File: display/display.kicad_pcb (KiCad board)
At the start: 2 copper layers, 177 x 107.2 mm, 19 parts, among them J1 DIN41612_03x32_ABC

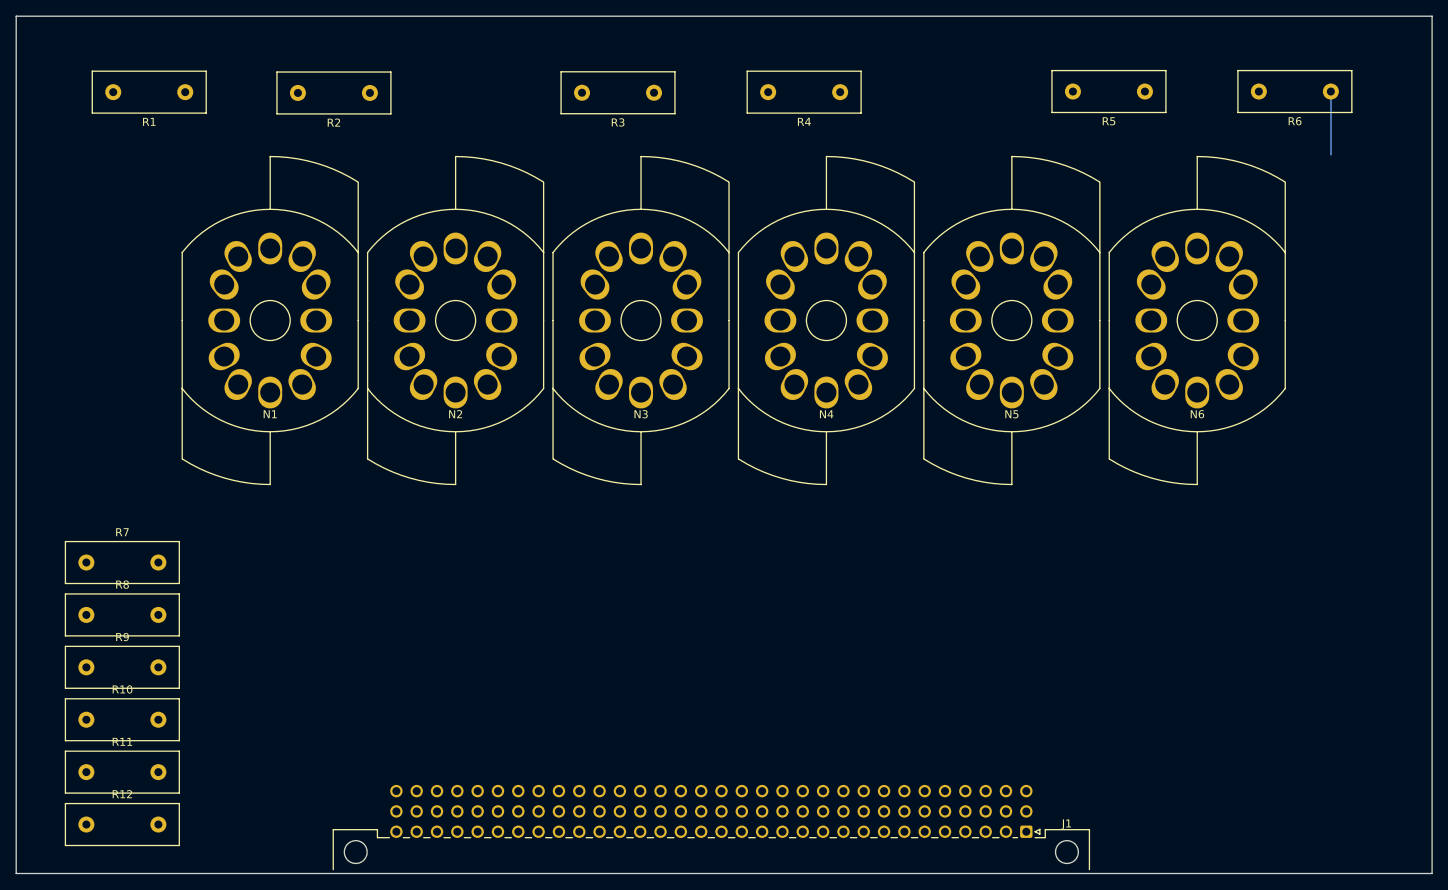
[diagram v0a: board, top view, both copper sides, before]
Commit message: Ongoing development
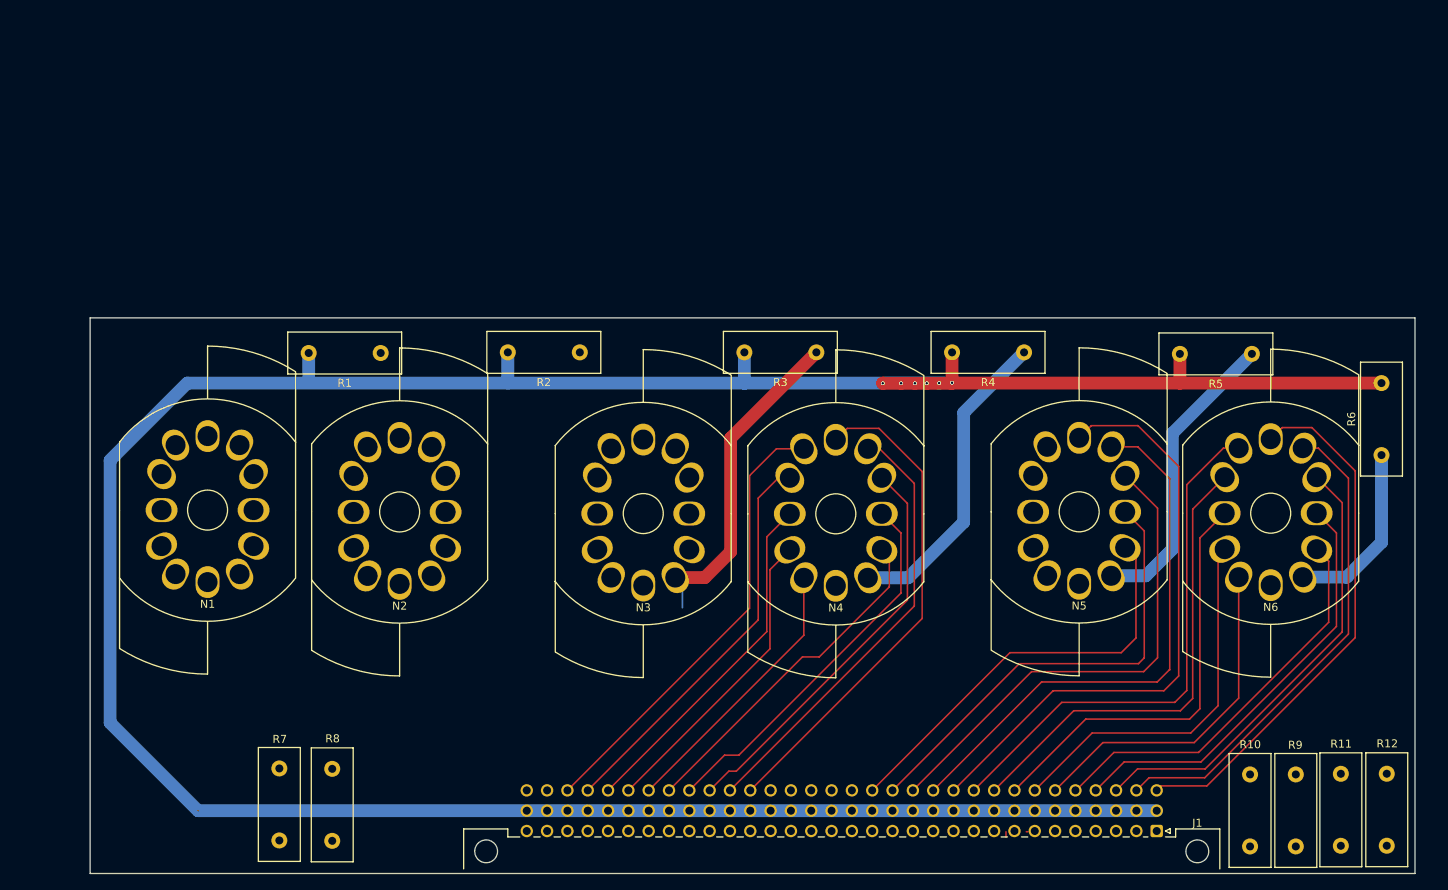
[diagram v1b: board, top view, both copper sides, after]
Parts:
- moved R12 162.7 mm to (225.5, 114.8), turned to -90 degrees
- moved R11 156.8 mm to (219.8, 114.8), turned to -90 degrees
- moved R9 151.8 mm to (214.1, 114.9), turned to -90 degrees
- moved R10 145.6 mm to (208.4, 114.9), turned to -90 degrees
- moved R6 45.9 mm to (224.8, 74.9), turned to 90 degrees
- moved R2 41.7 mm to (124.6, 62.1)
- moved R1 40.7 mm to (99.7, 62.2)
- moved R4 39.8 mm to (180.2, 62.1)
- moved R3 38.3 mm to (154.2, 62.1)
- moved R8 36.3 mm to (93.7, 114.2), turned to -90 degrees
- moved R5 35.4 mm to (208.6, 62.3)
- moved R7 35.3 mm to (87.1, 114.1), turned to -90 degrees
- moved N6 25.8 mm to (211.0, 82.2)
- moved N5 25.3 mm to (187.0, 82.0)
- moved N1 25.0 mm to (78.1, 81.8)
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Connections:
- J1 pad c11: /T5-9 -> /T5-6
- J1 pad c12: /T5-8 -> /T5-7
- J1 pad c13: /T5-7 -> /T5-8
- J1 pad c14: /T5-6 -> /T5-9
- J1 pad c15: /T5-5 -> /T5-0
- J1 pad c16: /T5-4 -> /T5-1
- J1 pad c17: /T5-3 -> /T5-2
- J1 pad c18: /T5-2 -> /T5-3
- J1 pad c19: /T5-1 -> /T5-4
- J1 pad c20: /T5-0 -> /T5-5
- J1 pad c21: /T4-9 -> /T4-6
- J1 pad c22: /T4-8 -> /T4-7
- J1 pad c23: /T4-7 -> /T4-8
- J1 pad c24: /T4-6 -> /T4-9
- J1 pad c25: /T4-5 -> /T4-0
- J1 pad c26: /T4-4 -> /T4-1
- J1 pad c27: /T4-3 -> /T4-2
- J1 pad c28: /T4-2 -> /T4-3
- J1 pad c29: /T4-1 -> /T4-4
- J1 pad c30: /T4-0 -> /T4-5
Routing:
- net Net-(J1-Pin_b1): track 0.00 -> 357.8 mm, vias 0 -> 6
- net /T5-6: track 0.00 -> 75.5 mm
- net /T5-7: track 0.00 -> 68.7 mm
- net /T6-6: track 0.00 -> 67.0 mm
- net /T6-5: track 0.00 -> 65.9 mm
- net /T6-7: track 0.00 -> 62.6 mm
- net /T4-6: track 0.00 -> 62.4 mm
- net /T5-8: track 0.00 -> 61.9 mm
- net /T6-4: track 0.00 -> 58.9 mm
- net /T5-9: track 0.00 -> 57.6 mm
- net /T6-8: track 0.00 -> 57.1 mm
- net /T4-5: track 0.00 -> 56.9 mm
- net /T4-7: track 0.00 -> 55.5 mm
- net /T6-9: track 0.00 -> 55.0 mm
- net /T6-3: track 0.00 -> 53.1 mm
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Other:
- board size 177 x 107.2 mm -> 165.6 x 69.5 mm
